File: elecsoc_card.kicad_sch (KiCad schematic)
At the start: 35 parts, among them J1 Conn_01x02_Pin, J2 Conn_01x02_Pin, U1 NA555D

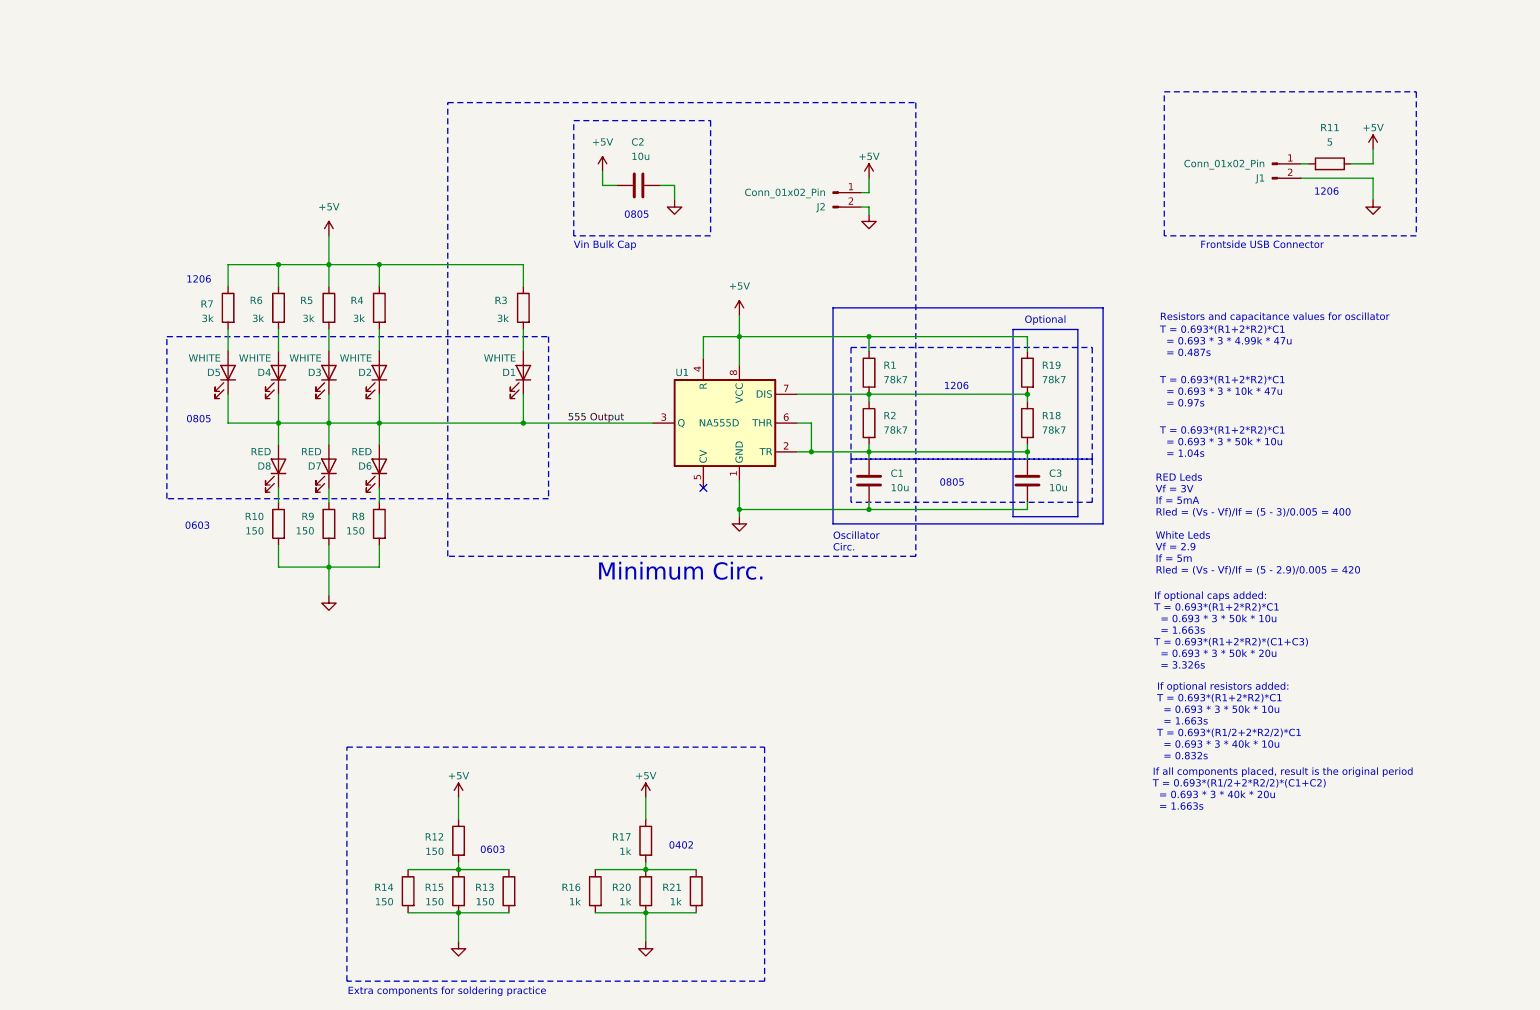
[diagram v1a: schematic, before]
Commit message: PCB finished plus gerbers
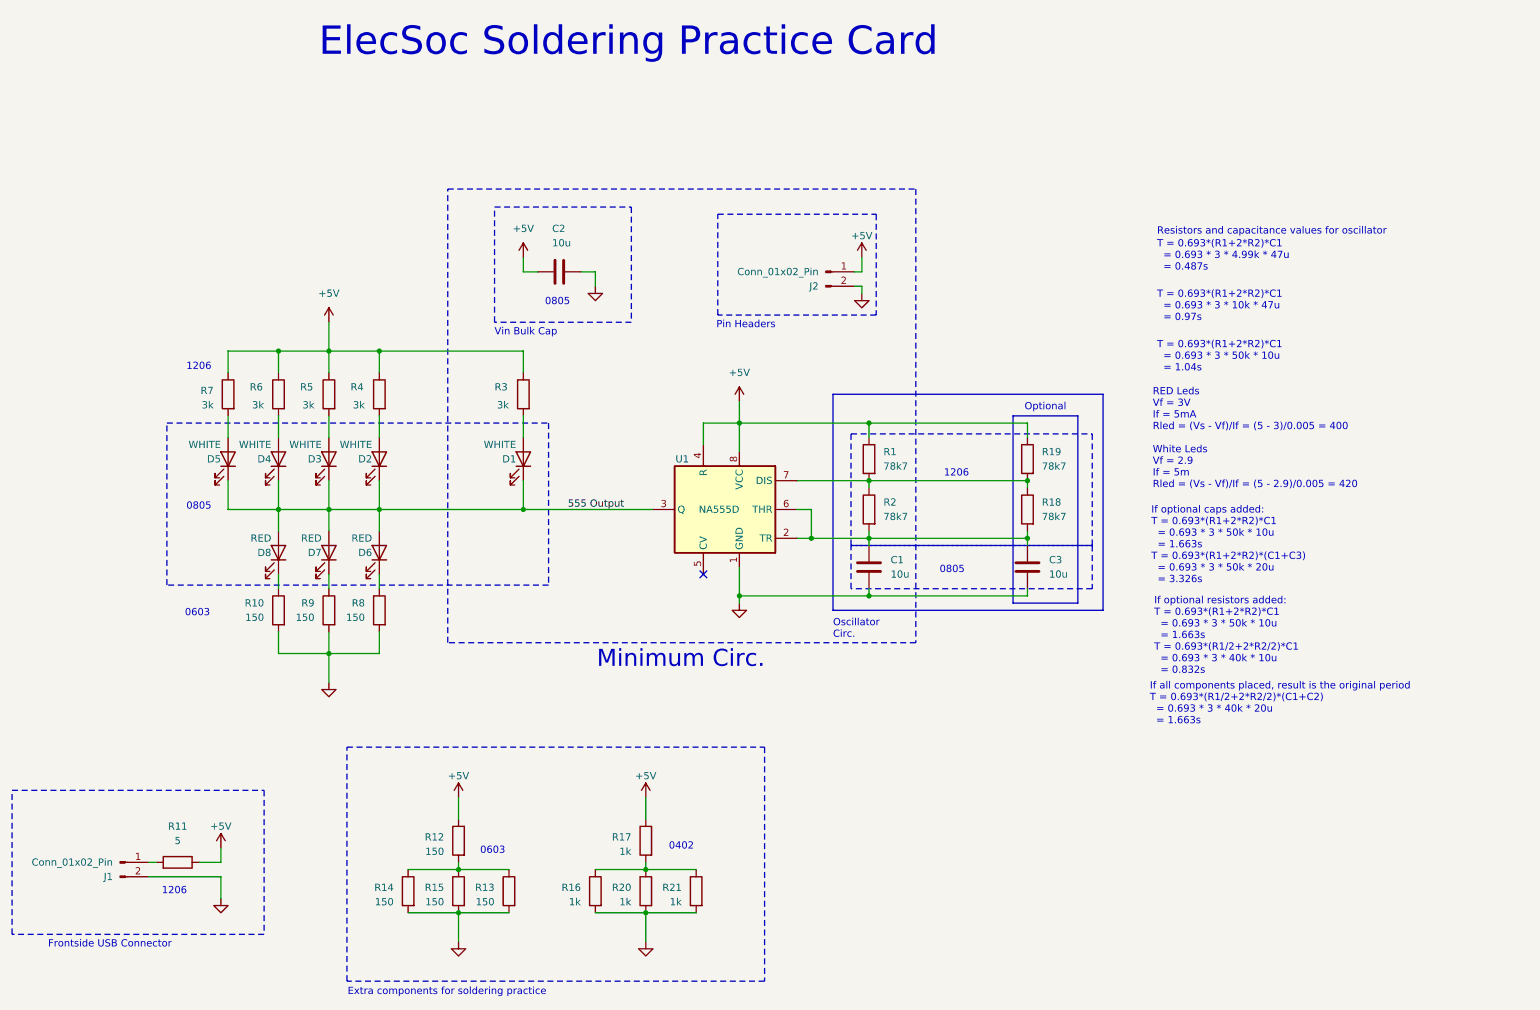
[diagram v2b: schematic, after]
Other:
- note added: "ElecSoc Soldering Practice Card"
- note added: "Pin Headers"
- moved on the sheet: C1, C2, C3, D1, D2, D3, D4, D5, D6, D7, D8, J1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

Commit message: BOM generated
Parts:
- C1, C2, C3: MPN (none) -> CL21A106KPFNNNF
- D1, D2, D3, D5: MPN (none) -> SMLMN2WB1CW1; Mfr. No. SMLMN2WB1CW1 -> (none)
- D4: MPN (none) -> SMLMN2WB1CW1; Mfr. No SMLMN2WB1CW1 -> (none)
- D6, D7: MPN (none) -> IN-S85AT5UW; Mfr. No. IN-S85AT5UW -> (none)
- D8: MPN (none) -> IN-S85AT5UW; Mfr. No: IN-S85AT5UW -> (none)
- J1: now left out of the parts list
- J2: MPN (none) -> 826632-1
- R1, R18, R19, R2: MPN (none) -> RT1206FRE0778K7L
- R10, R12, R13, R14, R15, R8, R9: MPN (none) -> MCT06030C1500FP500
- R11: MPN (none) -> RT1206FRD075R1L
- R16, R17, R20, R21: MPN (none) -> MCS04020C1001FE000
- R3, R4, R5, R6, R7: MPN (none) -> RT1206FRE073KL
- U1: MPN (none) -> 621-NE555S-13; Mfr. No: 621-NE555S-13 -> (none)
